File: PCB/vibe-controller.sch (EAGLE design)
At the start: 59 parts, among them J1 TRS Jack, J2 TRS Jack, Q1 SI2302CDS, Q2 SI2302CDS, Q3 ON Semi NTS4173P, SW2 MOM (OFF)-ON, SW3 MOM (OFF)-ON, SW4 MOM (OFF)-ON, SW5 MOM (OFF)-ON, SW6 MOM (OFF)-ON, SW7 MOM (OFF)-ON

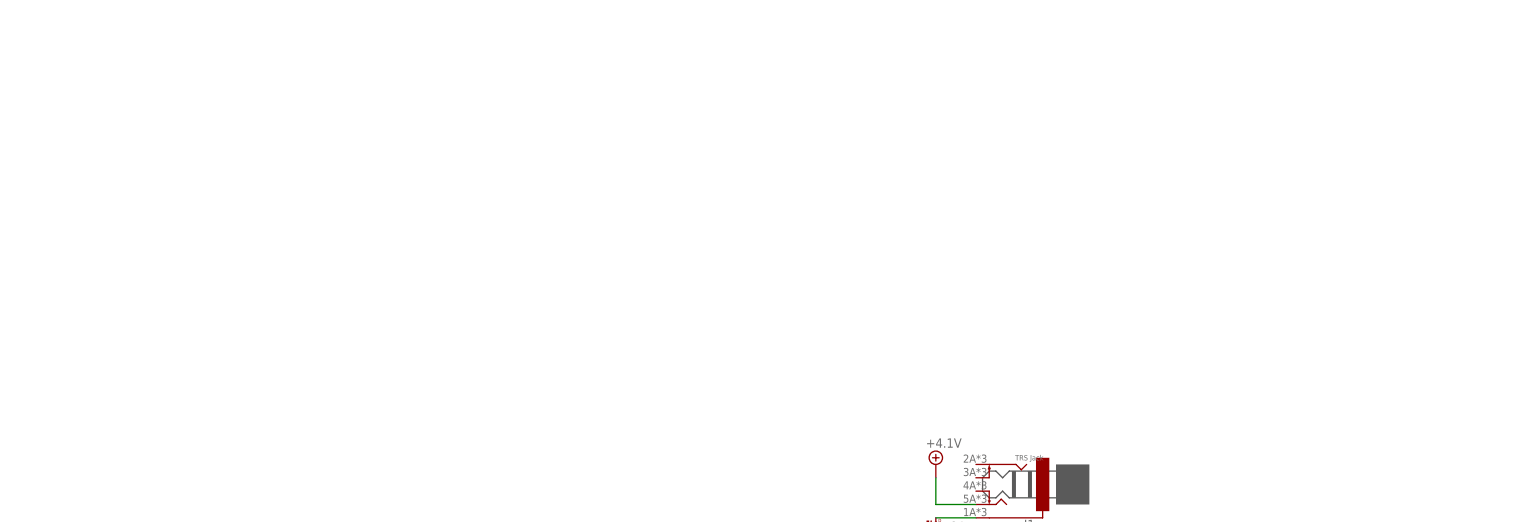
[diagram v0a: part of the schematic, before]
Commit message: Build notes
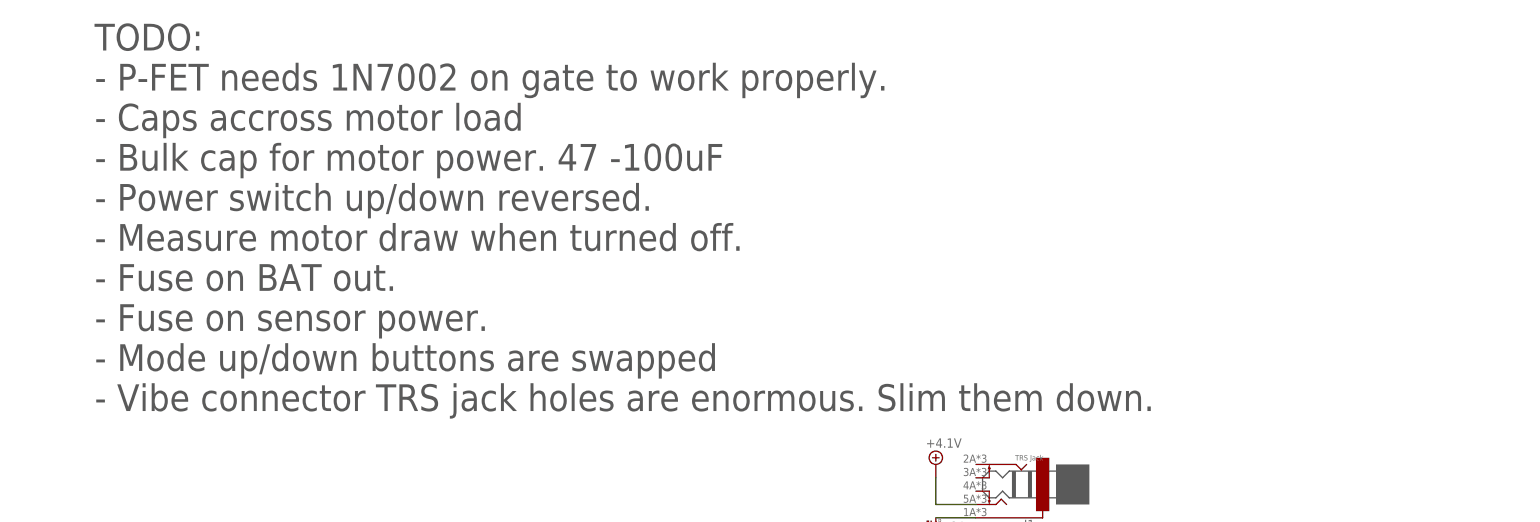
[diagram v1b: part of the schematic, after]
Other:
- note added: "TODO: - P-FET needs 1N7002 on gate to work properly. - Caps accross motor load - Bulk cap for motor power. 47 -100uF - Power switch up/down reversed. - Measure motor draw when turned off. - Fuse on BAT out. - Fuse on sensor power. - Mode up/down buttons are swapped - Vibe connector TRS jack holes are enormous. Slim them down."
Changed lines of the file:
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@@
 <text x="93.726" y="123.698" size="1.27" layer="97">GPIO #26</text>
 <text x="93.726" y="126.238" size="1.27" layer="97">GPIO #25</text>
+<text x="55.88" y="185.42" size="5.08" layer="97">TODO:
+- P-FET needs 1N7002 on gate to work properly.
+- Caps accross motor load
+- Bulk cap for motor power. 47 -100uF
+- Power switch up/down reversed.
+- Measure motor draw when turned off.
+- Fuse on BAT out.
+- Fuse on sensor power.
+- Mode up/down buttons are swapped
+- Vibe connector TRS jack holes are enormous. Slim them down.
+</text>
 </plain>
 <instances>
@@
 </drawing>
 <compatibility>
+<note version="6.3" minversion="6.2.2" severity="warning">
+Since Version 6.2.2 text objects can contain more than one line,
+which will not be processed correctly with this version.
+</note>
 <note version="8.2" severity="warning">
 Since Version 8.2, EAGLE supports online libraries. The ids
